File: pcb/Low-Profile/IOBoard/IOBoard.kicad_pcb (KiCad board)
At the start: 2 copper layers, 49.7 x 38 mm, 11 parts, among them J1 XT30PW-M, J3 Mounting holes, J4 DNP, J6 FH41-40S-0.5SH_05_

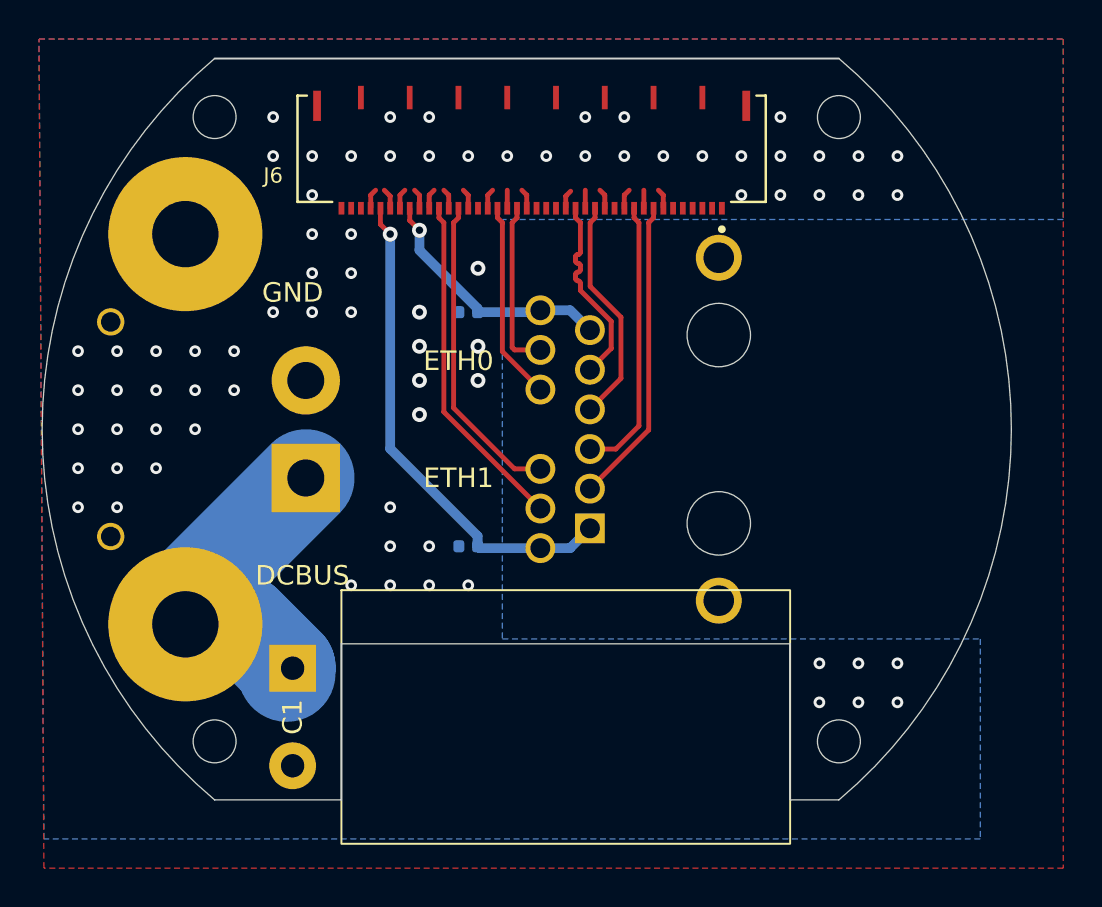
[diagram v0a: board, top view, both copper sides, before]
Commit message: Finished new 2+2 IOboard
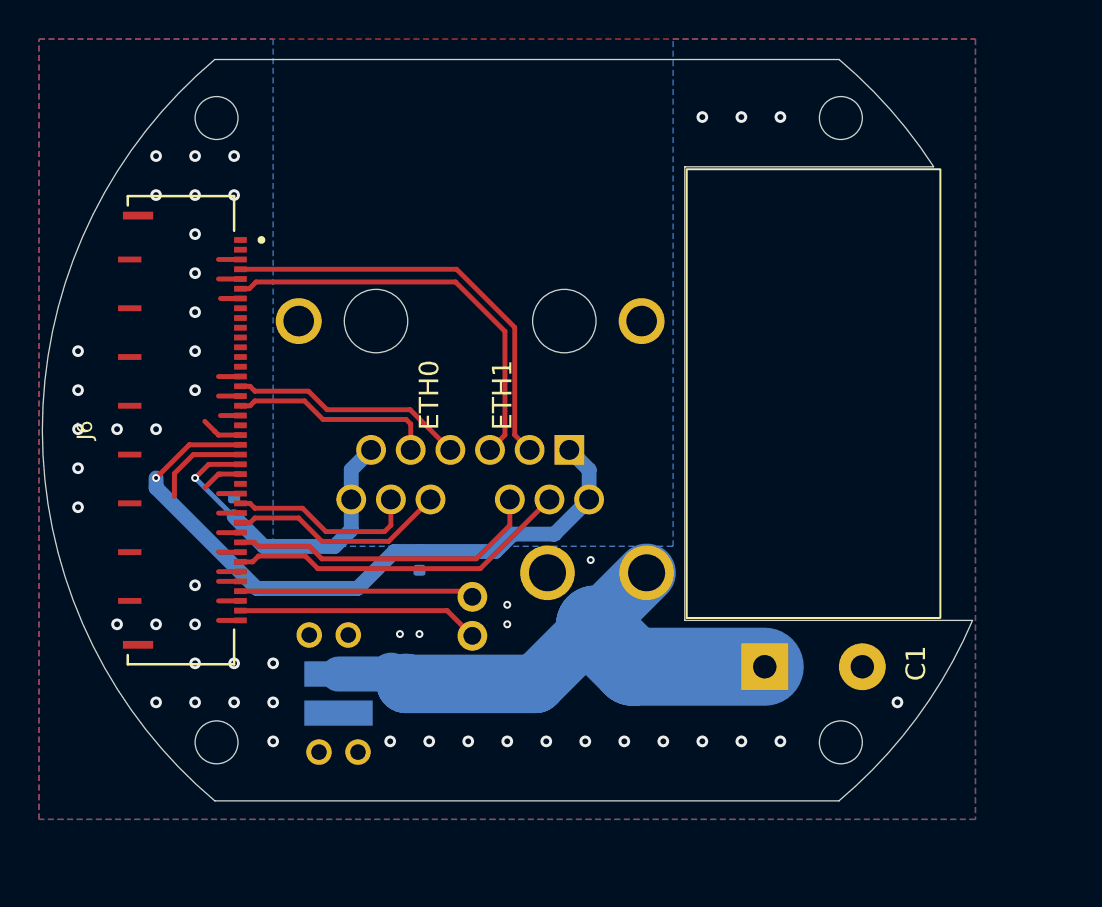
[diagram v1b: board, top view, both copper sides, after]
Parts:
- removed J3: Mounting holes, holes:Dual Post
- added U1: ~, Connector_AMASS:CONN-TH_4P-XT30PW-M, B.Cu at (151.7, 109.0)
- J1: value XT30PW-M -> UMPS-02-03.5-G-V-S-W-TR; footprint Connector_AMASS:AMASS_XT30PW-M_1x02_P2.50mm_Horizontal -> UMPS:SAMTEC_UMPS-02-03.5-G-V-S-W-TR
- moved C1 26.8 mm to (164.7, 112.2), turned to 90 degrees
- moved J6 22.9 mm to (132.3, 100.0), turned to -90 degrees
- moved C3 15.6 mm to (135.0, 104.0), turned to -90 degrees
- moved J4 13.9 mm to (147.1, 94.5), turned to 180 degrees
- moved J1 11.2 mm to (140.3, 113.5)
- moved C4 2.61 mm to (144.5, 106.8), turned to 90 degrees
- moved H1 0.11 mm to (134.1, 84.0)
- moved H2 0.11 mm to (166.1, 84.0)
- moved H3 0.11 mm to (134.1, 116.0)
- moved H4 0.11 mm to (166.1, 116.0)
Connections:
- J6 pad 10: /ETH1_RX_P -> GND
- J6 pad 14: /ETH0_TX_P -> GND
- J6 pad 16: /ETH0_TX_N -> /ETH0_TX_P
- J6 pad 18: GND -> /ETH0_TX_N
- J6 pad 22: /ETH0_RX_P -> /ETH1_CT1
- J6 pad 24: /ETH0_RX_N -> /ETH0_CT1
- J6 pad 28: /ETH1_TX_N -> /ETH0_RX_P
- J6 pad 30: /ETH1_TX_P -> /ETH0_RX_N
- J6 pad 32: GND -> /ETH1_TX_N
- J6 pad 33: /ETH0_CT1 -> GND
- J6 pad 34: GND -> /ETH1_TX_P
- J6 pad 36: /ETH1_CT1 -> GND
- J6 pad 37: GND -> /CAN_H
- J6 pad 39: GND -> /CAN_L
- J6 pad 4: GND -> /ETH1_RX_N
- J6 pad 41: SHIELD -> GND
- J6 pad 42: SHIELD -> GND
- J6 pad 43: SHIELD -> GND
- J6 pad 44: SHIELD -> GND
- J6 pad 45: SHIELD -> GND
- J6 pad 46: SHIELD -> GND
- J6 pad 47: SHIELD -> GND
- J6 pad 48: SHIELD -> GND
- J6 pad 49: SHIELD -> GND
- J6 pad 50: SHIELD -> GND
- J6 pad 6: GND -> /ETH1_RX_P
- J6 pad 8: /ETH1_RX_N -> GND
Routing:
- net /CAN_L: track 0.00 -> 12.4 mm
- net /CAN_H: track 0.00 -> 12.0 mm
- net DCBUS: track 16.5 -> 27.8 mm
- net /ETH1_CT1: track 25.6 -> 34.7 mm
- net GND: track 16.1 -> 24.7 mm, vias 75 -> 50
- net /ETH1_RX_P: track 14.3 -> 21.1 mm
- net /ETH1_RX_N: track 15.7 -> 21.9 mm
- net /ETH0_CT1: track 13.0 -> 16.9 mm
- net /ETH0_RX_N: track 10.2 -> 11.2 mm
- net /ETH0_RX_P: track 8.74 -> 9.77 mm
- net /ETH0_TX_N: track 10.0 -> 10.6 mm
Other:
- board size 49.7 x 38 mm -> 47.7 x 38 mm
- board text removed: "DCBUS"
- board text removed: "GND"
